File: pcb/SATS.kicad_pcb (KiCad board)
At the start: 2 copper layers, 27 parts, among them J1 Raspberry_Pi_2_3, J10 EXT_GPIO, J11 EXT_GPIO, J12 EXT_GPIO, J13 EXT_GPIO, J2 A00-432-262-450, J3 AudioJack4_SwitchTR1, J4 5V, J5 3.3V, J6 Card LED, J7 Wiegand, J8 Beep, J9 Card Power, SW1 Main Door Switch, SW2 Serv Door Switch, SW3 Third Reed Switch, U1 MCP23017_SP, U2 MCP23017_SP, U3 CD40109BE, U4 IRLZ14PBF

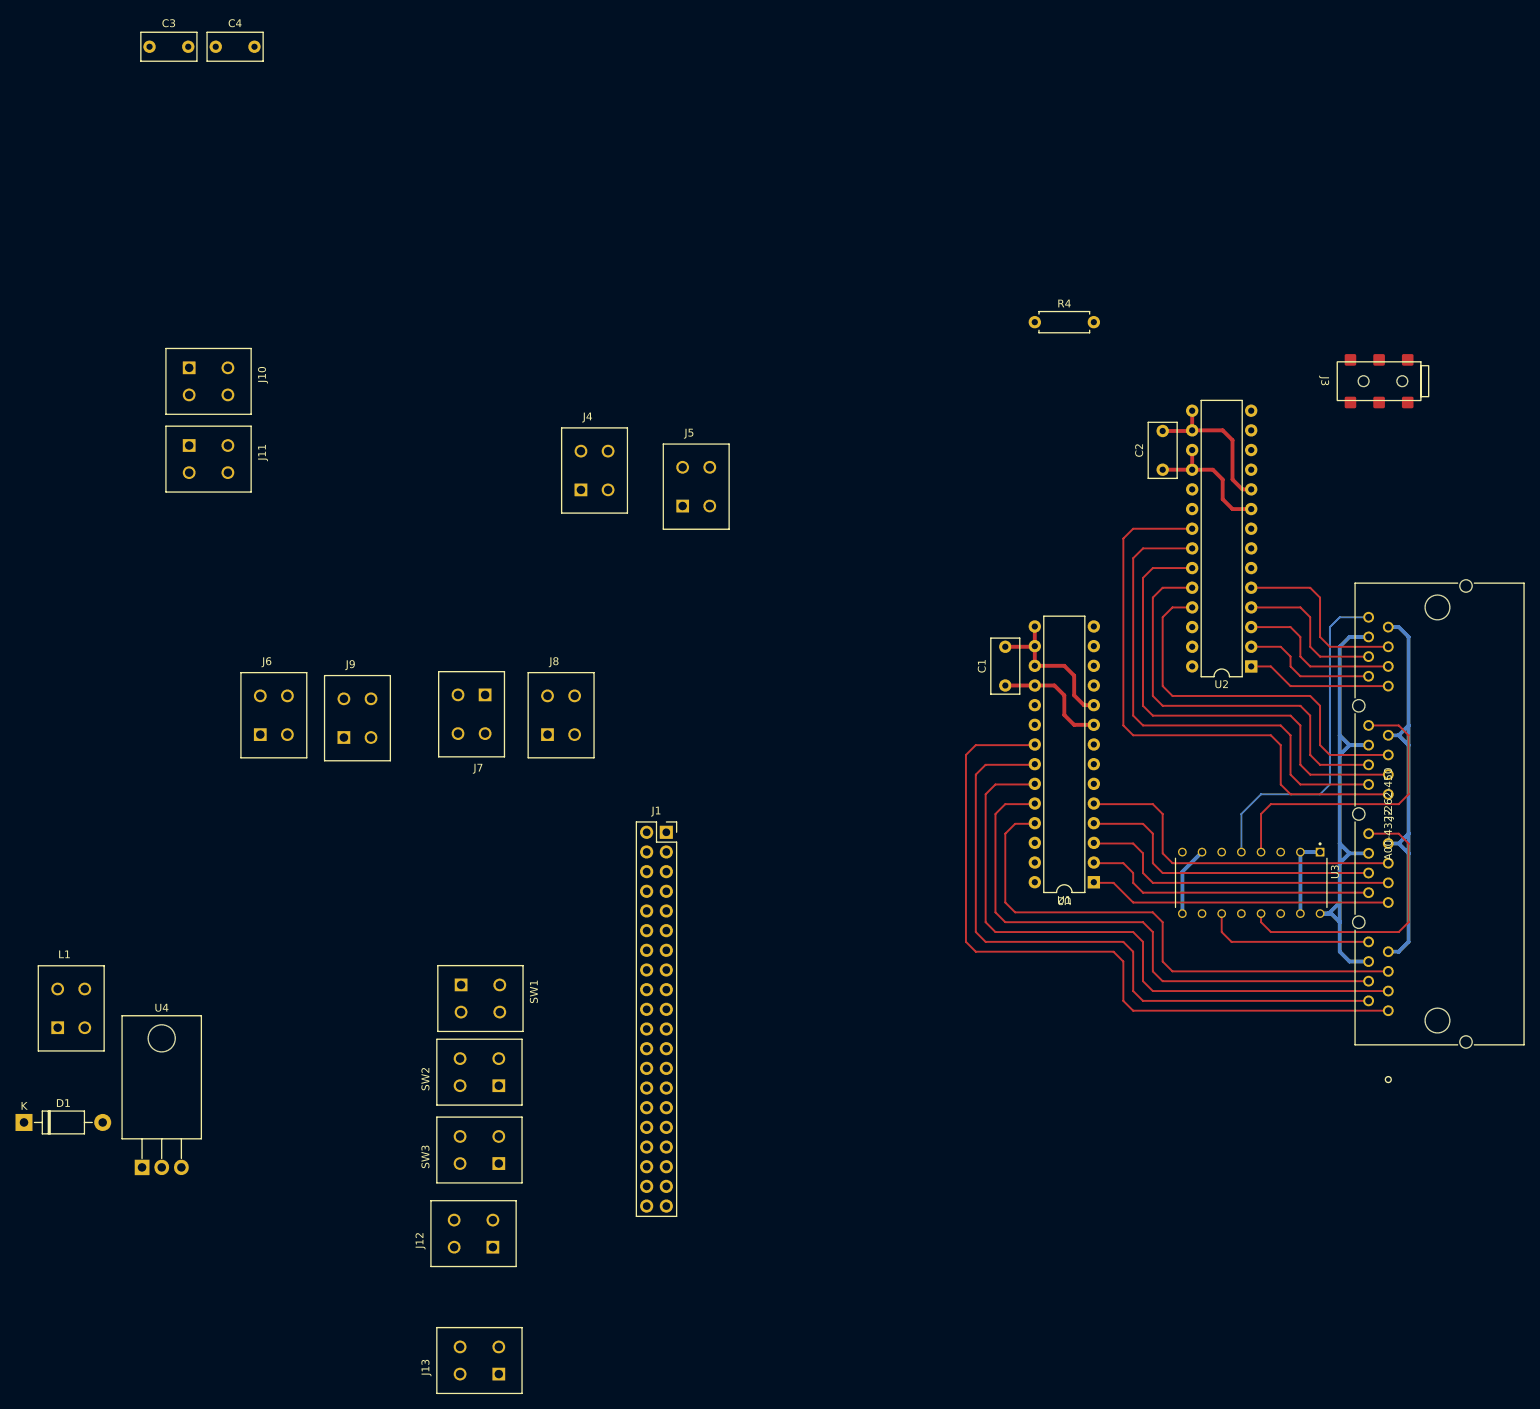
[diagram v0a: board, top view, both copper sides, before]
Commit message: mostly done
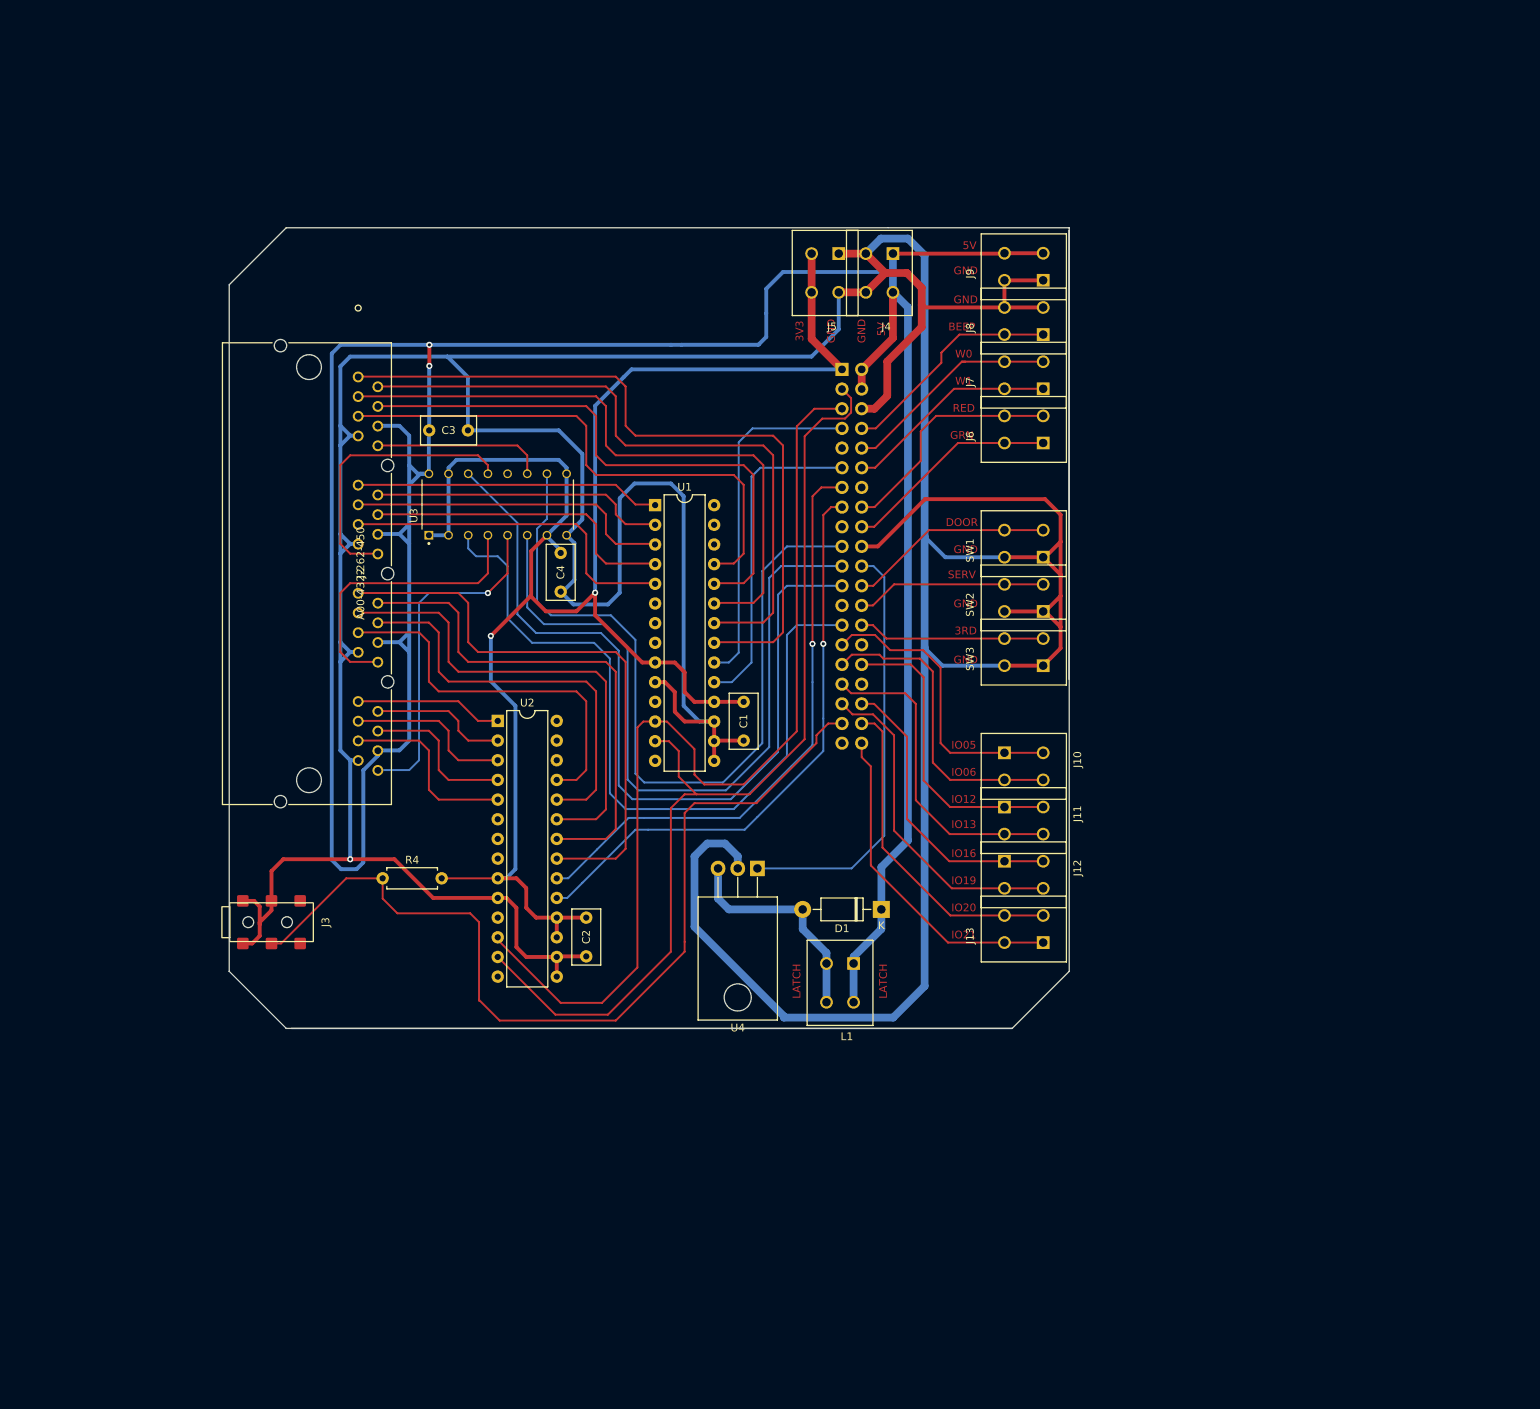
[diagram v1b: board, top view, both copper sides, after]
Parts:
- J1: moved to B.Cu
- moved J3 159.1 mm to (55.1, 134.6), turned to 90 degrees
- moved J2 156.2 mm to (66.3, 64.2), turned to -90 degrees
- moved J10 116.4 mm to (152.2, 114.5)
- moved J11 115.1 mm to (152.2, 121.5)
- moved D1 114.1 mm to (133.9, 133.0), turned to 180 degrees
- moved R4 110.7 mm to (69.5, 129.0)
- moved U3 108.9 mm to (84.3, 80.7), turned to 90 degrees
- moved J9 103.9 mm to (152.2, 50.0), turned to 90 degrees
- moved J6 103.6 mm to (152.2, 71.0), turned to 90 degrees
- moved L1 99.3 mm to (128.5, 142.5), turned to 180 degrees
- moved U2 97.5 mm to (84.3, 108.6), turned to 0 degrees
- moved SW3 95.2 mm to (152.2, 99.8)
- moved C2 94.3 mm to (95.8, 134.0), turned to -90 degrees
- moved SW2 93.2 mm to (152.2, 92.8)
- moved SW1 91.5 mm to (152.2, 85.8), turned to 90 degrees
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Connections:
- J1 pad 19: LED Sig1 -> LED Sig2
- J1 pad 21: LED Sig2 -> LED Sig4
- J1 pad 23: LED Sig3 -> LED Sig1
- J1 pad 27: LED Sig4 -> LED Sig3
- J11 pad 1: EXT_GPIO13 -> EXT_GPIO12
- J11 pad 2: EXT_GPIO13 -> EXT_GPIO12
- J11 pad 3: EXT_GPIO19 -> EXT_GPIO13
- J11 pad 4: EXT_GPIO19 -> EXT_GPIO13
- J12 pad 3: EXT_GPIO12 -> EXT_GPIO19
- J12 pad 4: EXT_GPIO12 -> EXT_GPIO19
- J7 pad 1: Wiegand 0 -> Wiegand 1
- J7 pad 2: Wiegand 0 -> Wiegand 1
- J7 pad 3: Wiegand 1 -> Wiegand 0
- J7 pad 4: Wiegand 1 -> Wiegand 0
- J9 pad 1: +5V -> Earth
- J9 pad 2: +5V -> Earth
- J9 pad 3: Earth -> +5V
- J9 pad 4: Earth -> +5V
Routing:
- net Earth: track 95.8 -> 669.9 mm, vias 0 -> 1
- net +5V: track 66.1 -> 384.8 mm, vias 0 -> 2
- net +3V3: track 52.1 -> 228.0 mm, vias 0 -> 2
- net SCL: track 0.00 -> 129.8 mm
- net SDA: track 0.00 -> 128.3 mm
- net 1-Wire: track 0.00 -> 119.3 mm
- net LED Sig1: track 0.00 -> 106.1 mm
- net LED Sig2: track 0.00 -> 101.8 mm
- net LED Sig3: track 0.00 -> 97.0 mm
- net LED Sig4: track 0.00 -> 94.6 mm
- net Int 2A: track 0.00 -> 76.6 mm, vias 0 -> 1
- net Int 2B: track 0.00 -> 75.6 mm, vias 0 -> 1
- net Latch: track 0.00 -> 55.0 mm
- net Int 1A: track 0.00 -> 45.0 mm
- net EXT_GPIO19: track 0.00 -> 43.0 mm
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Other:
- board outline added: 108.5 x 103.4 mm
- board text added: "3RD"
- board text added: "3V3"
- board text added: "5V"
- board text added: "BEEP"
- board text added: "DOOR"
- board text added: "GND"
- board text added: "GRN"
- board text added: "IO05"
- board text added: "IO06"
- board text added: "IO12"
- board text added: "IO13"
- board text added: "IO16"
- board text added: "IO19"
- board text added: "IO20"
- board text added: "IO21"
- board text added: "LATCH"
- board text added: "RED"
- board text added: "SERV"
- board text added: "W0"
- board text added: "W1"
- board text removed: "U2"
